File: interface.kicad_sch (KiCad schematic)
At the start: 42 parts, among them CN1 A1251WV-8P, CN2 B2B-PH-K-S, CN3 PH-3A_C2908624, U10 DRV8848PWPR, U18 2.00mm-4P-JST, U2 2.00mm-4P-JST, U21 TCA9534PWR, U22 PZ2.54-2*4, U7 ESP32-S3-WROOM-1, U8 LSM6DSOXTR

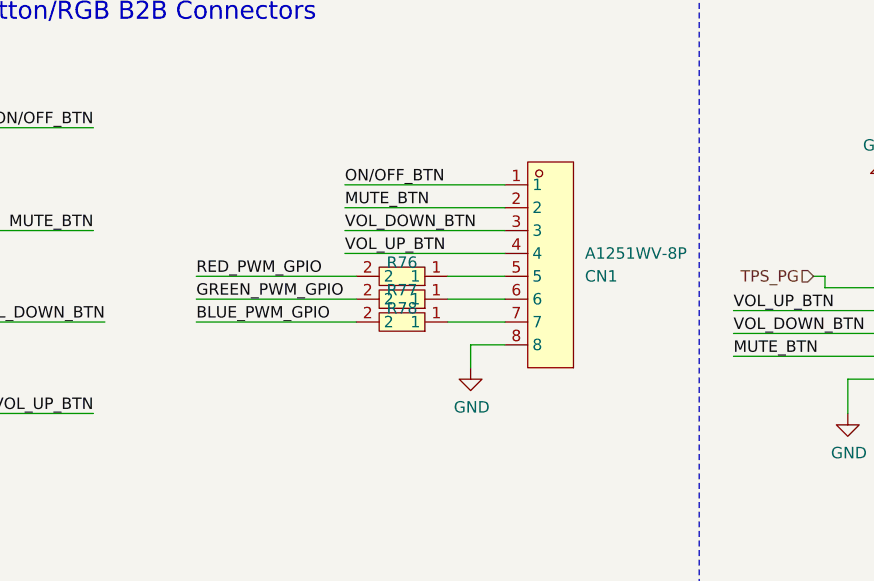
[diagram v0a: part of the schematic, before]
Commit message: 1
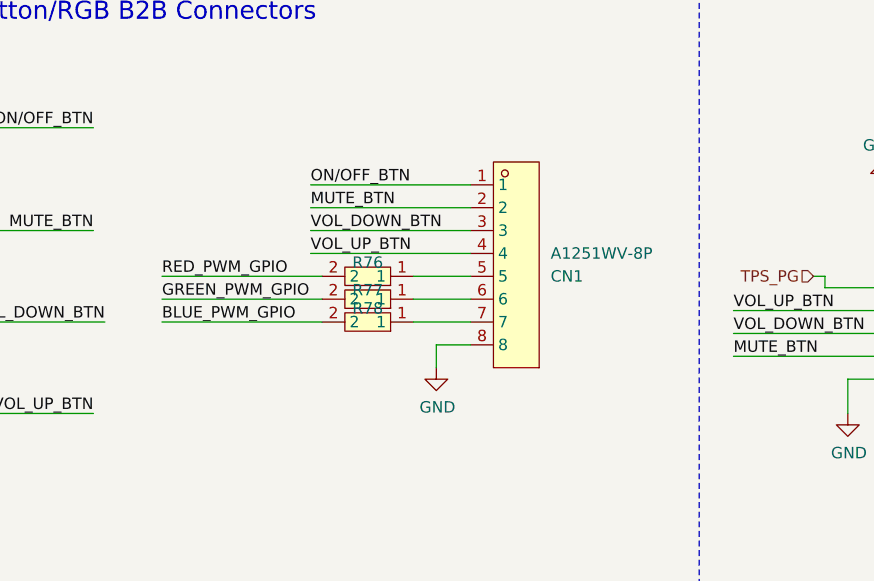
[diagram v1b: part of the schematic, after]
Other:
- moved on the sheet: CN1, R76, R77, R78
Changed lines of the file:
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@@
 	(wire
 		(pts
-			(xy 116.84 248.92) (xy 116.84 251.46)
+			(xy 113.03 248.92) (xy 113.03 251.46)
 		)
 		(stroke
@@
 	(wire
 		(pts
-			(xy 102.87 238.76) (xy 120.65 238.76)
+			(xy 99.06 238.76) (xy 116.84 238.76)
 		)
 		(stroke
@@
 	(wire
 		(pts
-			(xy 114.3 241.3) (xy 120.65 241.3)
+			(xy 110.49 241.3) (xy 116.84 241.3)
 		)
 		(stroke
@@
 	(wire
 		(pts
-			(xy 86.36 246.38) (xy 104.14 246.38)
+			(xy 82.55 246.38) (xy 100.33 246.38)
 		)
 		(stroke
@@
 	(wire
 		(pts
-			(xy 102.87 236.22) (xy 120.65 236.22)
+			(xy 99.06 236.22) (xy 116.84 236.22)
 		)
 		(stroke
@@
 	(wire
 		(pts
-			(xy 86.36 243.84) (xy 104.14 243.84)
+			(xy 82.55 243.84) (xy 100.33 243.84)
 		)
 		(stroke
@@
 	(wire
 		(pts
-			(xy 114.3 243.84) (xy 120.65 243.84)
+			(xy 110.49 243.84) (xy 116.84 243.84)
 		)
 		(stroke
@@
 	(wire
 		(pts
-			(xy 116.84 248.92) (xy 120.65 248.92)
+			(xy 113.03 248.92) (xy 116.84 248.92)
 		)
 		(stroke
@@
 	(wire
 		(pts
-			(xy 86.36 241.3) (xy 104.14 241.3)
+			(xy 82.55 241.3) (xy 100.33 241.3)
 		)
 		(stroke
@@
 	(wire
 		(pts
-			(xy 102.87 233.68) (xy 120.65 233.68)
+			(xy 99.06 233.68) (xy 116.84 233.68)
 		)
 		(stroke
@@
 	(wire
 		(pts
-			(xy 102.87 231.14) (xy 120.65 231.14)
+			(xy 99.06 231.14) (xy 116.84 231.14)
 		)
 		(stroke
@@
 	(wire
 		(pts
-			(xy 114.3 246.38) (xy 120.65 246.38)
+			(xy 110.49 246.38) (xy 116.84 246.38)
 		)
 		(stroke
@@
 	)
 	(label "RED_PWM_GPIO"
-		(at 86.36 241.3 0)
+		(at 82.55 241.3 0)
 		(effects
 			(font
@@
 	)
 	(label "VOL_UP_BTN"
-		(at 102.87 238.76 0)
+		(at 99.06 238.76 0)
 		(effects
 			(font
@@
 	)
 	(label "VOL_DOWN_BTN"
-		(at 102.87 236.22 0)
+		(at 99.06 236.22 0)
 		(effects
 			(font
@@
 	)
 	(label "GREEN_PWM_GPIO"
-		(at 86.36 243.84 0)
+		(at 82.55 243.84 0)
 		(effects
 			(font
@@
 	)
 	(label "MUTE_BTN"
-		(at 102.87 233.68 0)
+		(at 99.06 233.68 0)
 		(effects
 			(font
@@
 	)
 	(label "BLUE_PWM_GPIO"
-		(at 86.36 246.38 0)
+		(at 82.55 246.38 0)
 		(effects
 			(font
@@
 	)
 	(label "ON{slash}OFF_BTN"
-		(at 102.87 231.14 0)
+		(at 99.06 231.14 0)
 		(effects
 			(font
@@
 	(symbol
 		(lib_id "JLSC:0603WAF1500T5E")
-		(at 109.22 241.3 180)
+		(at 105.41 241.3 180)
 		(unit 1)
 		(body_style 1)
@@
 		(dnp no)
 		(property "Reference" "R76"
-			(at 109.22 239.776 0)
+			(at 105.41 239.776 0)
 			(show_name no)
 			(do_not_autoplace no)
@@
 		)
 		(property "Value" "0603WAF1500T5E"
-			(at 109.22 245.11 0)
+			(at 105.41 245.11 0)
 			(hide yes)
 			(show_name no)
@@
 		)
 		(property "Footprint" "EasyEDA:R0603"
-			(at 109.22 233.68 0)
+			(at 105.41 233.68 0)
 			(hide yes)
 			(show_name no)
@@
 		)
 		(property "Datasheet" "https://lcsc.com/product-detail/Chip-Resistor-Surface-Mount-UniOhm_150R-1500-1_C22808.html"
-			(at 109.22 231.14 0)
+			(at 105.41 231.14 0)
 			(hide yes)
 			(show_name no)
@@
 		)
 		(property "Description" "150Ω (1500) ±1%"
-			(at 109.22 241.3 0)
+			(at 105.41 241.3 0)
 			(hide yes)
 			(show_name no)
@@
 		)
 		(property "Manufacturer" "UNI-ROYAL(厚声)"
-			(at 109.22 228.6 0)
+			(at 105.41 228.6 0)
 			(hide yes)
 			(show_name no)
@@
 		)
 		(property "MPN" "0603WAF1500T5E"
-			(at 109.22 226.06 0)
+			(at 105.41 226.06 0)
 			(hide yes)
 			(show_name no)
@@
 		)
 		(property "LCSC Part" "C22808"
-			(at 109.22 223.52 0)
+			(at 105.41 223.52 0)
 			(hide yes)
 			(show_name no)
@@
 	(symbol
 		(lib_id "power:GND")
-		(at 116.84 251.46 0)
+		(at 113.03 251.46 0)
 		(unit 1)
 		(body_style 1)
@@
 		(dnp no)
 		(property "Reference" "#PWR0162"
-			(at 116.84 257.81 0)
+			(at 113.03 257.81 0)
 			(hide yes)
 			(show_name no)
@@
 		)
 		(property "Value" "GND"
-			(at 116.967 255.8542 0)
+			(at 113.157 255.8542 0)
 			(show_name no)
 			(do_not_autoplace no)
@@
 		)
 		(property "Footprint" ""
-			(at 116.84 251.46 0)
+			(at 113.03 251.46 0)
 			(hide yes)
 			(show_name no)
@@
 		)
 		(property "Datasheet" ""
-			(at 116.84 251.46 0)
+			(at 113.03 251.46 0)
 			(hide yes)
 			(show_name no)
@@
 		)
 		(property "Description" "Power symbol creates a global label with name \"GND\" , ground"
-			(at 116.84 251.46 0)
+			(at 113.03 251.46 0)
 			(hide yes)
 			(show_name no)
@@
 	(symbol
 		(lib_id "JLSC:A1251WV-8P")
-		(at 124.46 240.03 270)
+		(at 120.65 240.03 270)
 		(mirror x)
 		(unit 1)
@@
 		(dnp no)
 		(property "Reference" "CN1"
-			(at 129.54 241.3001 90)
+			(at 125.73 241.3001 90)
 			(show_name no)
 			(do_not_autoplace no)
@@
 		)
 		(property "Value" "A1251WV-8P"
-			(at 129.54 238.7601 90)
+			(at 125.73 238.7601 90)
 			(show_name no)
 			(do_not_autoplace no)
@@
 		)
 		(property "Footprint" "EasyEDA:CONN-TH_8P-P1.25_A1251WV-8P"
-			(at 113.03 240.03 0)
+			(at 109.22 240.03 0)
 			(hide yes)
 			(show_name no)
@@
 		)
 		(property "Datasheet" "https://lcsc.com/product-detail/Connectors_Changjiang-Connectors-A1251WV-8P_C225096.html"
-			(at 110.49 240.03 0)
+			(at 106.68 240.03 0)
 			(hide yes)
 			(show_name no)
@@
 		)
 		(property "Description" ""
-			(at 124.46 240.03 0)
+			(at 120.65 240.03 0)
 			(hide yes)
 			(show_name no)
@@
 		)
 		(property "Manufacturer" "CJT(长江连接器)"
-			(at 107.95 240.03 0)
+			(at 104.14 240.03 0)
 			(hide yes)
 			(show_name no)
@@
 		)
 		(property "MPN" "A1251WV-8P"
-			(at 105.41 240.03 0)
+			(at 101.6 240.03 0)
 			(hide yes)
 			(show_name no)
@@
 		)
 		(property "LCSC Part" "C225096"
-			(at 102.87 240.03 0)
+			(at 99.06 240.03 0)
 			(hide yes)
 			(show_name no)
@@
 	(symbol
 		(lib_id "JLSC:0603WAF1500T5E")
-		(at 109.22 243.84 180)
+		(at 105.41 243.84 180)
 		(unit 1)
 		(body_style 1)
@@
 		(dnp no)
 		(property "Reference" "R77"
-			(at 109.22 242.824 0)
+			(at 105.41 242.824 0)
 			(show_name no)
 			(do_not_autoplace no)
@@
 		)
 		(property "Value" "0603WAF1500T5E"
-			(at 109.22 247.65 0)
+			(at 105.41 247.65 0)
 			(hide yes)
 			(show_name no)
@@
 		)
 		(property "Footprint" "EasyEDA:R0603"
-			(at 109.22 236.22 0)
+			(at 105.41 236.22 0)
 			(hide yes)
 			(show_name no)
@@
 		)
 		(property "Datasheet" "https://lcsc.com/product-detail/Chip-Resistor-Surface-Mount-UniOhm_150R-1500-1_C22808.html"
-			(at 109.22 233.68 0)
+			(at 105.41 233.68 0)
 			(hide yes)
 			(show_name no)
@@
 		)
 		(property "Description" "150Ω (1500) ±1%"
-			(at 109.22 243.84 0)
+			(at 105.41 243.84 0)
 			(hide yes)
 			(show_name no)
@@
 		)
 		(property "Manufacturer" "UNI-ROYAL(厚声)"
-			(at 109.22 231.14 0)
+			(at 105.41 231.14 0)
 			(hide yes)
 			(show_name no)
@@
 		)
 		(property "MPN" "0603WAF1500T5E"
-			(at 109.22 228.6 0)
+			(at 105.41 228.6 0)
 			(hide yes)
 			(show_name no)
@@
 		)
 		(property "LCSC Part" "C22808"
-			(at 109.22 226.06 0)
+			(at 105.41 226.06 0)
 			(hide yes)
 			(show_name no)
@@
 	(symbol
 		(lib_id "JLSC:0603WAF3300T5E")
-		(at 109.22 246.38 180)
+		(at 105.41 246.38 180)
 		(unit 1)
 		(body_style 1)
@@
 		(dnp no)
 		(property "Reference" "R78"
-			(at 109.22 244.856 0)
+			(at 105.41 244.856 0)
 			(show_name no)
 			(do_not_autoplace no)
@@
 		)
 		(property "Value" "0603WAF3300T5E"
-			(at 109.22 250.19 0)
+			(at 105.41 250.19 0)
 			(hide yes)
 			(show_name no)
@@
 		)
 		(property "Footprint" "EasyEDA:R0603"
-			(at 109.22 238.76 0)
+			(at 105.41 238.76 0)
 			(hide yes)
 			(show_name no)
@@
 		)
 		(property "Datasheet" "https://lcsc.com/product-detail/Chip-Resistor-Surface-Mount-UniOhm_330R-3300-1_C23138.html"
-			(at 109.22 236.22 0)
+			(at 105.41 236.22 0)
 			(hide yes)
 			(show_name no)
@@
 		)
 		(property "Description" "330Ω (3300) ±1%"
-			(at 109.22 246.38 0)
+			(at 105.41 246.38 0)
 			(hide yes)
 			(show_name no)
@@
 		)
 		(property "Manufacturer" "UNI-ROYAL(厚声)"
-			(at 109.22 233.68 0)
+			(at 105.41 233.68 0)
 			(hide yes)
 			(show_name no)
@@
 		)
 		(property "MPN" "0603WAF3300T5E"
-			(at 109.22 231.14 0)
+			(at 105.41 231.14 0)
 			(hide yes)
 			(show_name no)
@@
 		)
 		(property "LCSC Part" "C23138"
-			(at 109.22 228.6 0)
+			(at 105.41 228.6 0)
 			(hide yes)
 			(show_name no)
